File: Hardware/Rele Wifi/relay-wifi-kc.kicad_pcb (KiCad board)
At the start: 2 copper layers, 101.6 x 81.5 mm, 47 parts, among them J1 SalidaRele1, J2 SalidaRele2, J3 SalidaRele3, J4 SalidaRele4, K1 RELAY_C, K2 RELAY_C, K3 RELAY_C, K4 RELAY_C, Q1 TO23, Q2 TO23, Q3 TO23, Q4 TO23, U1 LM78M05_TO220, U2 ESP32_DevKit_V1_DOIT, U3 PC817, U4 PC817, U5 PC817, U6 PC817

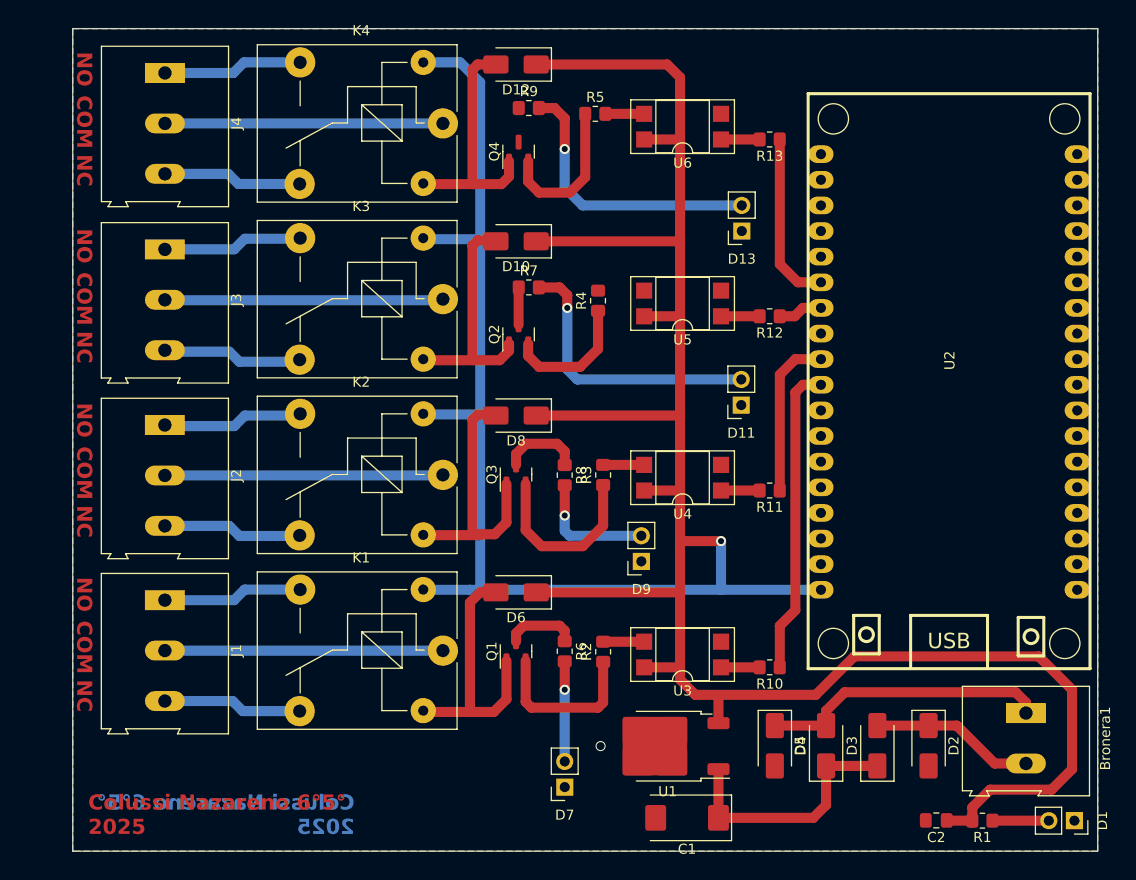
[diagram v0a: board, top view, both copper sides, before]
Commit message: Esquematico y PCB V4
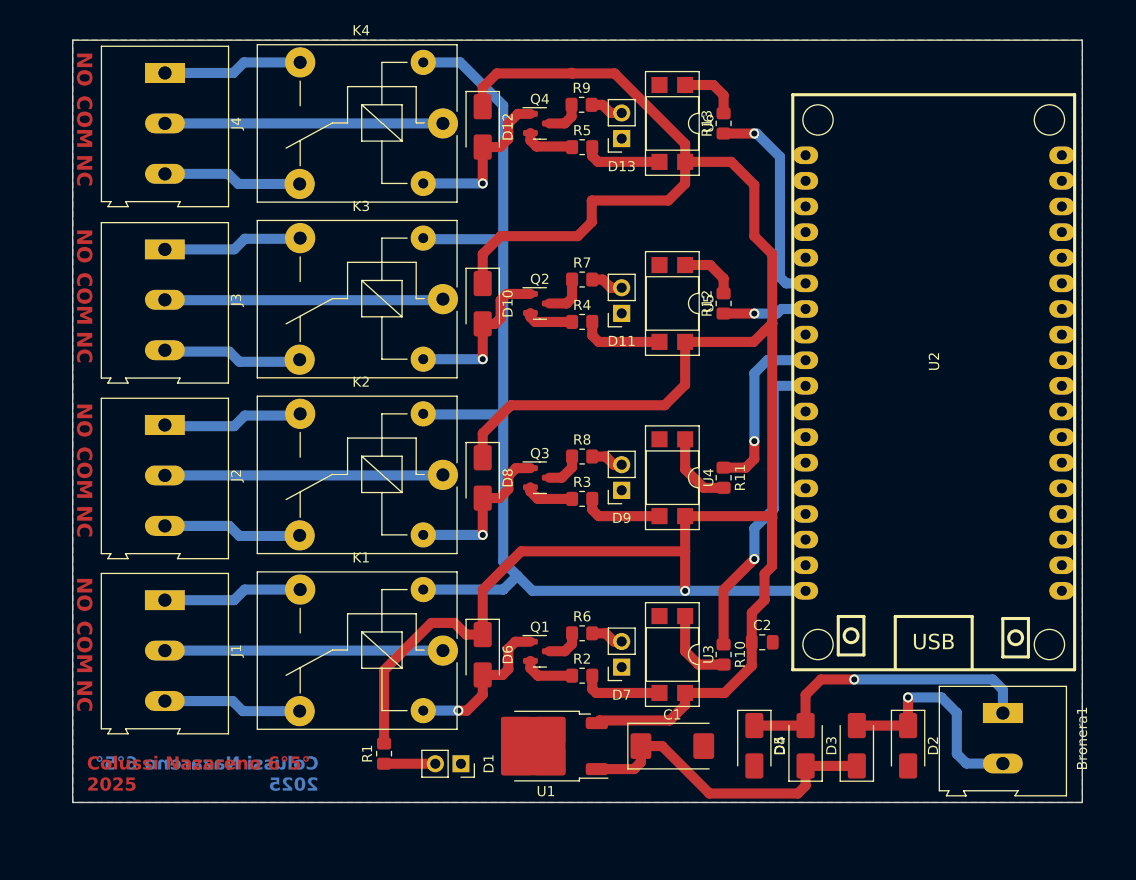
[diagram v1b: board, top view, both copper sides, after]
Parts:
- moved D1 61.1 mm to (65.9, 97.8)
- moved R1 59.7 mm to (58.3, 96.8), turned to 90 degrees
- moved C2 24.7 mm to (95.8, 85.7), turned to 0 degrees
- moved D13 15.0 mm to (81.8, 35.8)
- moved D11 14.9 mm to (81.8, 53.1)
- moved D7 13.2 mm to (81.8, 88.2)
- moved U1 12.1 mm to (74.3, 96.0)
- moved D9 7.31 mm to (81.8, 70.7)
- moved C1 7.26 mm to (86.9, 96.0), turned to 0 degrees
- moved D10 7.01 mm to (68.1, 52.2), turned to -90 degrees
- moved D12 7.01 mm to (68.1, 34.6), turned to -90 degrees
- moved D6 7.01 mm to (68.1, 87.0), turned to -90 degrees
- moved D8 7.01 mm to (68.1, 69.4), turned to -90 degrees
- moved R7 5.34 mm to (77.9, 49.8)
- moved R9 5.24 mm to (77.9, 32.4)
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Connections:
- net 5V renamed +5V
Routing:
- net +5V: track 316.7 -> 343.8 mm
- net Net-(D11-A): track 28.2 -> 3.26 mm, vias 1 -> 0
- net Net-(D13-A): track 28.1 -> 3.31 mm, vias 1 -> 0
- net Net-(Q3-B): track 17.8 -> 4.84 mm
- net Net-(D8-A): track 27.4 -> 16.3 mm, vias 0 -> 1
- net Net-(Q1-B): track 16.2 -> 5.16 mm
- net Net-(D6-A): track 26.6 -> 15.8 mm, vias 0 -> 1
- net Net-(Q4-B): track 15.1 -> 5.14 mm
- net Net-(D9-A): track 12.3 -> 3.26 mm, vias 1 -> 0
- net Net-(Q2-B): track 13.1 -> 4.73 mm
- net Net-(R4-Pad2): track 0.00 -> 8.28 mm
- net Net-(D12-A): track 24.4 -> 16.5 mm, vias 0 -> 1
- net Net-(D10-A): track 23.9 -> 16.4 mm, vias 0 -> 1
- net Net-(D3-K): track 25.0 -> 31.8 mm
- net Net-(D7-A): track 9.92 -> 3.26 mm, vias 1 -> 0
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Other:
- board size 101.6 x 81.5 mm -> 100.1 x 75.6 mm
